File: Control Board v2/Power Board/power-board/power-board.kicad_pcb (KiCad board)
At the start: 6 copper layers, 92 x 118.5 mm, 26 parts, among them J1 1366005, J2 1366005, J6 Conn_01x04, J7 Conn_01x02, SW1 SW_SPST, U2 MOC3083S-TA1

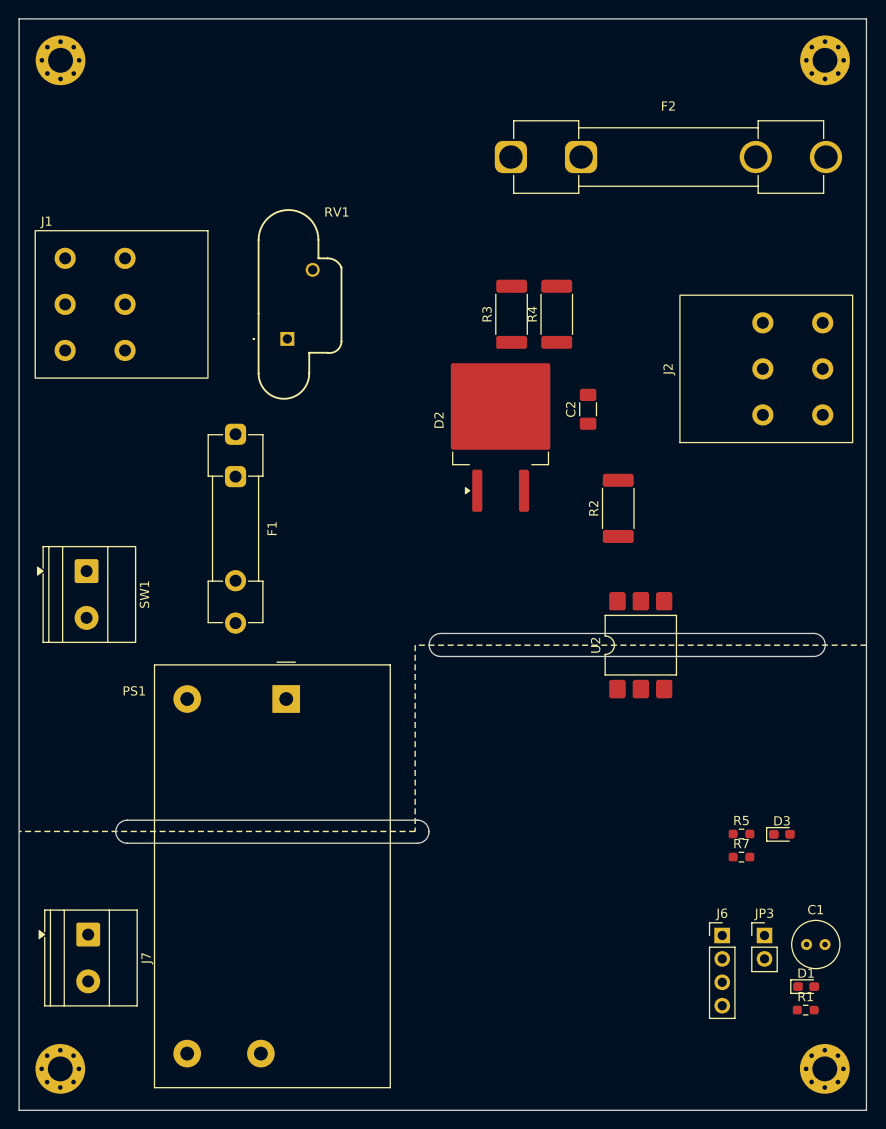
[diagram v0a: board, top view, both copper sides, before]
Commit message: PCB layout is generally complete
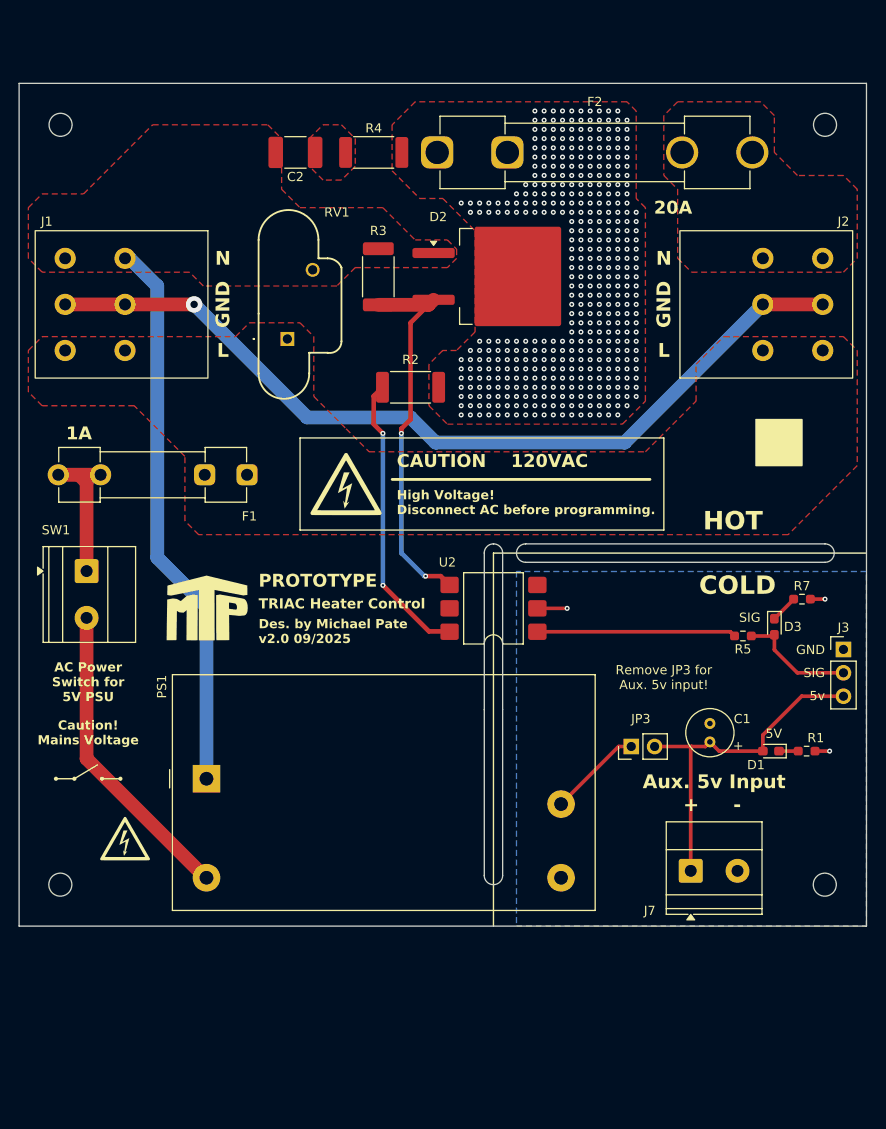
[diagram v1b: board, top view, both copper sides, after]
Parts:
- removed J6: Conn_01x04, Connector_PinHeader_2.54mm:PinHeader_1x04_P2.54mm_Vertical
- added G***: LOGO, LOGO, F.Cu at (149.0, 73.5)
- added G***: LOGO, LOGO, F.Cu at (125.0, 112.0)
- added G***: LOGO, LOGO, B.Cu at (147.5, 106.5)
- added G***: LOGO, LOGO, B.Cu at (178.5, 73.5)
- added J3: Conn_01x03, Connector_PinHeader_2.54mm:PinHeader_1x03_P2.54mm_Vertical, F.Cu at (203.0, 91.5)
- added REF**: MTP Logo 10mm Low Detail, Watermarks:MTP Logo 10mm Low Detail, F.Cu at (134.0, 87.0)
- C2: footprint Capacitor_SMD:C_1206_3216Metric_Pad1.33x1.80mm_HandSolder -> Capacitor_SMD:C_1812_4532Metric_Pad1.57x3.40mm_HandSolder
- H1, H2, H3, H4: footprint MountingHole:MountingHole_2.7mm_M2.5_Pad_Via -> MountingHole:MountingHole_2.5mm
- moved J7 65.8 mm to (186.4, 115.5), turned to 0 degrees
- moved C2 42.3 mm to (143.5, 37.5), turned to 180 degrees
- moved R7 28.8 mm to (198.5, 86.0)
- moved R1 28.1 mm to (199.0, 102.5)
- moved R4 26.5 mm to (152.0, 37.5), turned to 0 degrees
- moved R2 26.1 mm to (156.0, 63.0), turned to 0 degrees
- moved D1 25.9 mm to (195.1, 102.5), turned to 180 degrees
- moved JP3 25.1 mm to (180.0, 102.0), turned to 90 degrees
- moved C1 24.4 mm to (188.5, 101.5), turned to 90 degrees
- moved D3 22.6 mm to (195.5, 89.0), turned to -90 degrees
- moved R5 21.5 mm to (192.1, 90.0), turned to 180 degrees
- moved H3 20.0 mm to (118.0, 117.0)
- moved H4 20.0 mm to (201.0, 117.0)
- moved U2 16.5 mm to (165.0, 87.0), turned to 180 degrees
- moved D2 15.6 mm to (166.2, 51.0), turned to 0 degrees
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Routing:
- net GNDPWR: track 0.00 -> 94.7 mm, vias 0 -> 1
- net LN: track 0.00 -> 60.5 mm
- net /Project Architecture/Heater Control/LN_OPTO: track 0.00 -> 41.8 mm, vias 0 -> 2
- net VDD: track 0.00 -> 38.1 mm
- net /Project Architecture/Power Supply/L1_F1_SW: track 0.00 -> 33.7 mm
- net /Project Architecture/Heater Control/L1_F2_OPTO: track 0.00 -> 31.6 mm, vias 0 -> 2
- net /Project Architecture/Heater Control/D_R5_OPTO: track 0.00 -> 21.6 mm
- net /Project Architecture/Power Supply/L1_F1: track 0.00 -> 15.4 mm
- net D_Heater: track 0.00 -> 12.7 mm
- net /Project Architecture/Power Supply/VDD_AC_DC: track 0.00 -> 10.2 mm
- net GND: track 0.00 -> 6.41 mm, vias 0 -> 3
- net /Project Architecture/Heater Control/D3_K: track 0.00 -> 2.99 mm
- net /Project Architecture/Power Supply/D1_K: track 0.00 -> 2.09 mm
- net /Project Architecture/Heater Control/L1_F2: vias 0 -> 428
- added copper zone on F.Cu, net /Project Architecture/Heater Control/L1_F2
- added copper zone on F.Cu, net /Project Architecture/Heater Control/L1_F2_RC
- added copper zone on F.Cu, net /Project Architecture/Heater Control/L1_HEATER
- added copper zone on B.Cu, net GND
- added copper zone on F.Cu, net L1
- added copper zone on F.Cu, net LN
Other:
- board size 92 x 118.5 mm -> 92 x 91.5 mm
- copper layers 6 -> 2
- board text added: "+"
- board text added: "-"
- board text added: "1A"
- board text added: "20A"
- board text added: "5V"
- board text added: "5v"
- board text added: "AC Power Switch for 5V PSU"
- board text added: "Aux. 5v Input"
- board text added: "CAUTION 120VAC"
- board text added: "COLD"
- board text added: "Caution! Mains Voltage"
- board text added: "Des. by Michael Pate v2.0 09/2025"
- board text added: "GND"
- board text added: "HOT"
- board text added: "High Voltage! Disconnect AC before programming."
- board text added: "L"
- board text added: "N"
- board text added: "PROTOTYPE"
- board text added: "Remove JP3 for Aux. 5v input!"
- board text added: "SIG"
- board text added: "TRIAC Heater Control"
